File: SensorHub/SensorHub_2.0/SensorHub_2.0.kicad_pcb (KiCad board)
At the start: 2 copper layers, 1 part, among them U1 R7FA4E2B93CFM#AA0

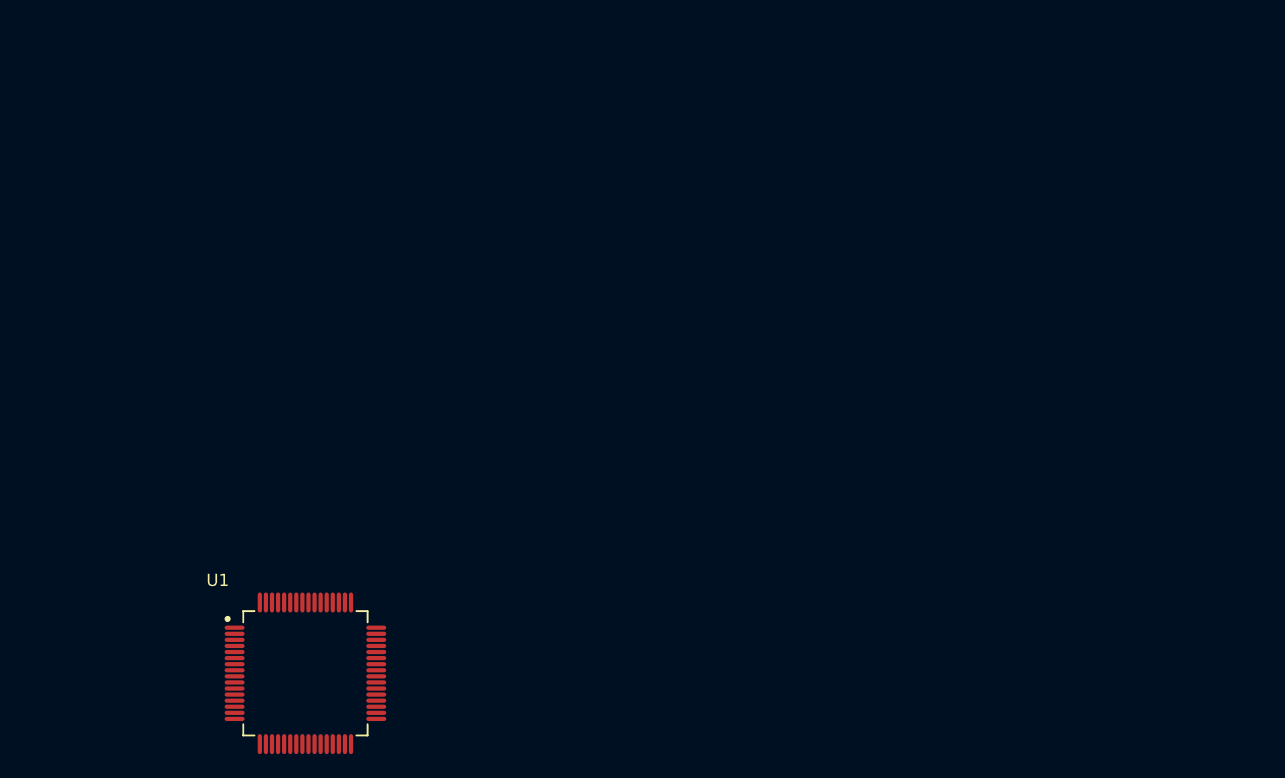
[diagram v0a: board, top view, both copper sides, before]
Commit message: 1st version SensorHub
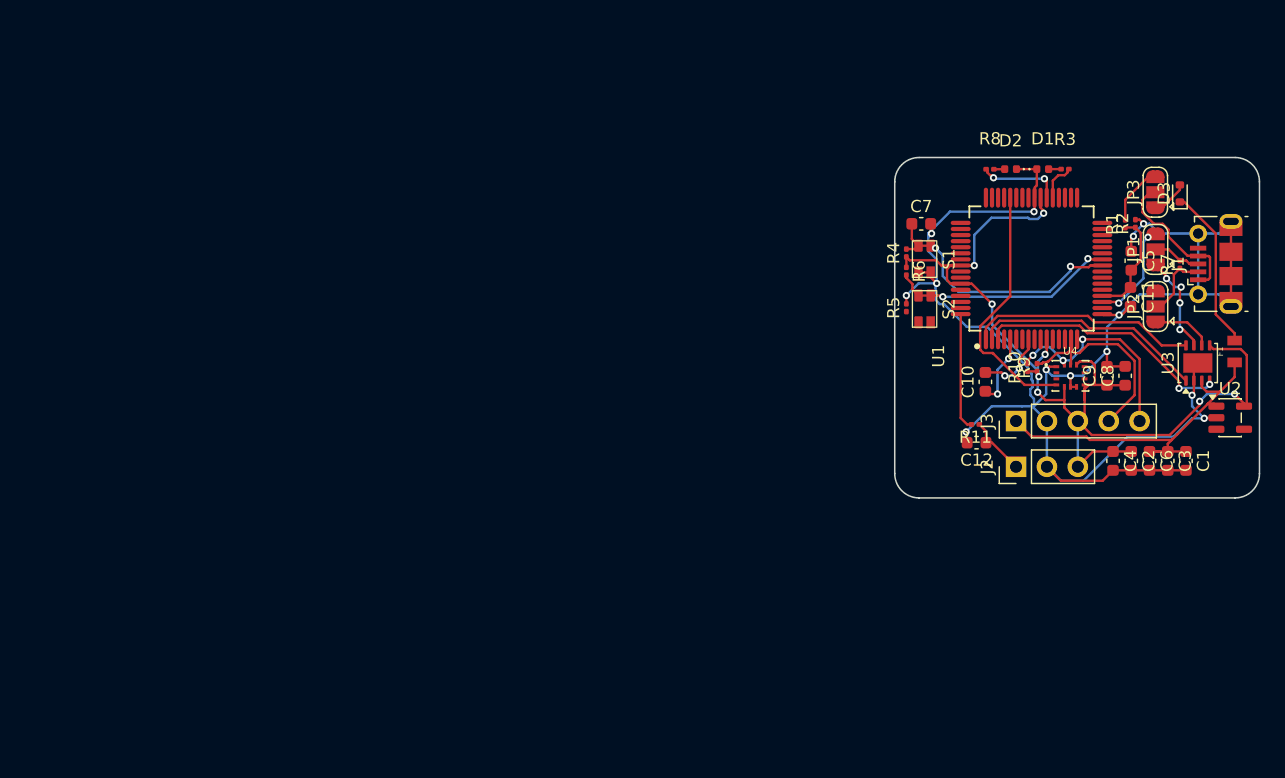
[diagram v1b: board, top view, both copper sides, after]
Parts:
- added C1: 10 uF, Capacitor_SMD:C_0603_1608Metric, F.Cu at (200.5, 120.0)
- added C10: 4.7 uF, Capacitor_SMD:C_0603_1608Metric, F.Cu at (184.0, 113.5)
- added C11: 0.1 uF, Capacitor_SMD:C_0603_1608Metric, F.Cu at (195.9, 106.5)
- added C12: 0.1 uF, Capacitor_SMD:C_0603_1608Metric, F.Cu at (183.3, 118.5)
- added C2: 10 uF, Capacitor_SMD:C_0603_1608Metric, F.Cu at (196.0, 120.0)
- added C3: 1 milF, Capacitor_SMD:C_0603_1608Metric, F.Cu at (199.0, 120.0)
- added C4: 1 milF, Capacitor_SMD:C_0603_1608Metric, F.Cu at (194.5, 120.0)
- added C5: 1 uF, Capacitor_SMD:C_0603_1608Metric, F.Cu at (196.0, 103.5)
- added C6: 0.1 uF, Capacitor_SMD:C_0603_1608Metric, F.Cu at (197.5, 120.0)
- added C7: 1 uF, Capacitor_SMD:C_0603_1608Metric, F.Cu at (178.7, 100.5)
- added C8: 0.1 uF, Capacitor_SMD:C_0603_1608Metric, F.Cu at (195.5, 113.0)
- added C9: 0.1 uF, Capacitor_SMD:C_0603_1608Metric, F.Cu at (194.0, 113.0)
- added D1: LED, LED_SMD:LED_0402_1005Metric, F.Cu at (188.7, 96.0)
- added D2: LED, LED_SMD:LED_0402_1005Metric, F.Cu at (186.1, 96.0)
- added D3: 1N4148WT, Diode_SMD:D_SOD-523, F.Cu at (200.0, 98.0)
- added F1: 6V 0.5A, SensorHub MicroMod Carrier v1.1.0b:0805, F.Cu at (204.5, 111.0)
- added J1: USB_B_Micro, Connector_USB:USB_Micro-B_Molex-105017-0001, F.Cu at (203.0, 103.8)
- added J2: Conn_01x03, Connector_PinHeader_2.54mm:PinHeader_1x03_P2.54mm_Vertical, F.Cu at (186.5, 120.5)
- added J3: Conn_01x05, Connector_PinHeader_2.54mm:PinHeader_1x05_P2.54mm_Vertical, F.Cu at (186.5, 116.7)
- added JP1: SolderJumper_3_Open, Jumper:SolderJumper-3_P1.3mm_Open_RoundedPad1.0x1.5mm, F.Cu at (198.0, 102.6)
- added JP2: SolderJumper_3_Open, Jumper:SolderJumper-3_P1.3mm_Open_RoundedPad1.0x1.5mm, F.Cu at (198.0, 107.3)
- added JP3: SolderJumper_3_Open, Jumper:SolderJumper-3_P1.3mm_Open_RoundedPad1.0x1.5mm, F.Cu at (198.0, 97.9)
- added R1: 15 K, Resistor_SMD:R_0201_0603Metric, F.Cu at (195.5, 100.5)
- added R10: 4.7 K, Resistor_SMD:R_0201_0603Metric, F.Cu at (187.5, 112.3)
- added R11: 1 K, Resistor_SMD:R_0201_0603Metric, F.Cu at (183.2, 117.0)
- added R2: 30 K, Resistor_SMD:R_0201_0603Metric, F.Cu at (196.3, 100.5)
- added R3: 1.33 K, Resistor_SMD:R_0201_0603Metric, F.Cu at (190.6, 96.0)
- added R4: 4.7 K, Resistor_SMD:R_0201_0603Metric, F.Cu at (177.5, 102.9)
- added R5: 1.5 K, Resistor_SMD:R_0201_0603Metric, F.Cu at (177.5, 107.4)
- added R6: 10 K, Resistor_SMD:R_0201_0603Metric, F.Cu at (177.5, 104.4)
- added R7: ~, Resistor_SMD:R_0201_0603Metric, F.Cu at (200.0, 103.8)
- added R8: 1.33 K, Resistor_SMD:R_0201_0603Metric, F.Cu at (184.4, 96.0)
- added R9: 4.7 K, Resistor_SMD:R_0201_0603Metric, F.Cu at (188.2, 112.3)
- added S1: Reset, Library:Button_Mini_2.5x1.7mm, F.Cu at (178.5, 103.4)
- added S2: Boot, Library:Button_Mini_2.5x1.7mm, F.Cu at (178.5, 107.5)
- added U$40: ROBOTPATIENT_SMALL_MODULEBOARD, RobotPatient_BMI270_v1.2_Feb2024:RP_SMALL_SENSOR_OUTLINE, F.Cu at (191.5, 109.0)
- added U2: AP2112K-3.3, Package_TO_SOT_SMD:SOT-23-5, F.Cu at (204.1, 116.5)
- added U3: TJA1051TK-3, Package_SON:HVSON-8-1EP_3x3mm_P0.65mm_EP1.6x2.4mm, F.Cu at (201.5, 112.0)
- added U4: BMI270, BMI270:XDCR_BMI270, F.Cu at (191.0, 113.0)
- moved U1 68.4 mm to (187.8, 104.2), turned to 90 degrees
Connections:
- U1 pad 1: unconnected-(U1-P400-Pad1) -> /Sleep
- U1 pad 11: unconnected-(U1-VCC-Pad11) -> +3.3V
- U1 pad 15: unconnected-(U1-P408-Pad15) -> /SCX
- U1 pad 16: unconnected-(U1-P407-Pad16) -> /SDX
- U1 pad 17: unconnected-(U1-VSS_USB-Pad17) -> GND
- U1 pad 18: unconnected-(U1-USB_DM-Pad18) -> /USB_DM
- U1 pad 19: unconnected-(U1-USB_DP-Pad19) -> /USB_DP
- U1 pad 2: unconnected-(U1-P401-Pad2) -> /TXD
- U1 pad 20: unconnected-(U1-VCC_USB-Pad20) -> /V_USB_Mic
- U1 pad 25: unconnected-(U1-~{RES}-Pad25) -> /RES
- U1 pad 26: unconnected-(U1-MD-Pad26) -> /Boot
- U1 pad 3: unconnected-(U1-CACREF-Pad3) -> /RXD
- U1 pad 37: unconnected-(U1-P112-Pad37) -> /P112
- U1 pad 38: unconnected-(U1-P113-Pad38) -> /P113
- U1 pad 39: unconnected-(U1-VCC-Pad39) -> +3.3V
- U1 pad 40: unconnected-(U1-VSS-Pad40) -> GND
- U1 pad 44: unconnected-(U1-P104-Pad44) -> /INT1
- U1 pad 5: unconnected-(U1-VCL-Pad5) -> /VCL
- U1 pad 56: unconnected-(U1-VREFH-Pad56) -> +3.3V
- U1 pad 59: unconnected-(U1-VREFH0-Pad59) -> +3.3V
- U1 pad 64: unconnected-(U1-P000-Pad64) -> /P000
- U1 pad 8: unconnected-(U1-VSS-Pad8) -> GND
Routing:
- net GND: track 0.00 -> 147.5 mm, vias 0 -> 15
- net +3.3V: track 0.00 -> 87.1 mm, vias 0 -> 8
- net +5V: track 0.00 -> 29.9 mm
- net /RES: track 0.00 -> 22.8 mm, vias 0 -> 2
- net /RXD: track 0.00 -> 21.3 mm, vias 0 -> 2
- net /INT1: track 0.00 -> 21.0 mm
- net /TXD: track 0.00 -> 19.2 mm
- net /SCX: track 0.00 -> 19.1 mm
- net /Sleep: track 0.00 -> 18.8 mm
- net /Boot: track 0.00 -> 18.7 mm, vias 0 -> 2
- net /SDX: track 0.00 -> 18.2 mm, vias 0 -> 3
- net Net-(D3-K): track 0.00 -> 13.5 mm
- net /V_usb: track 0.00 -> 12.9 mm
- net /P000: track 0.00 -> 9.65 mm
- net /V_USB_Mic: track 0.00 -> 8.91 mm
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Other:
- board outline added: 30 x 28 mm

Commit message: MYRGM080200C41RA
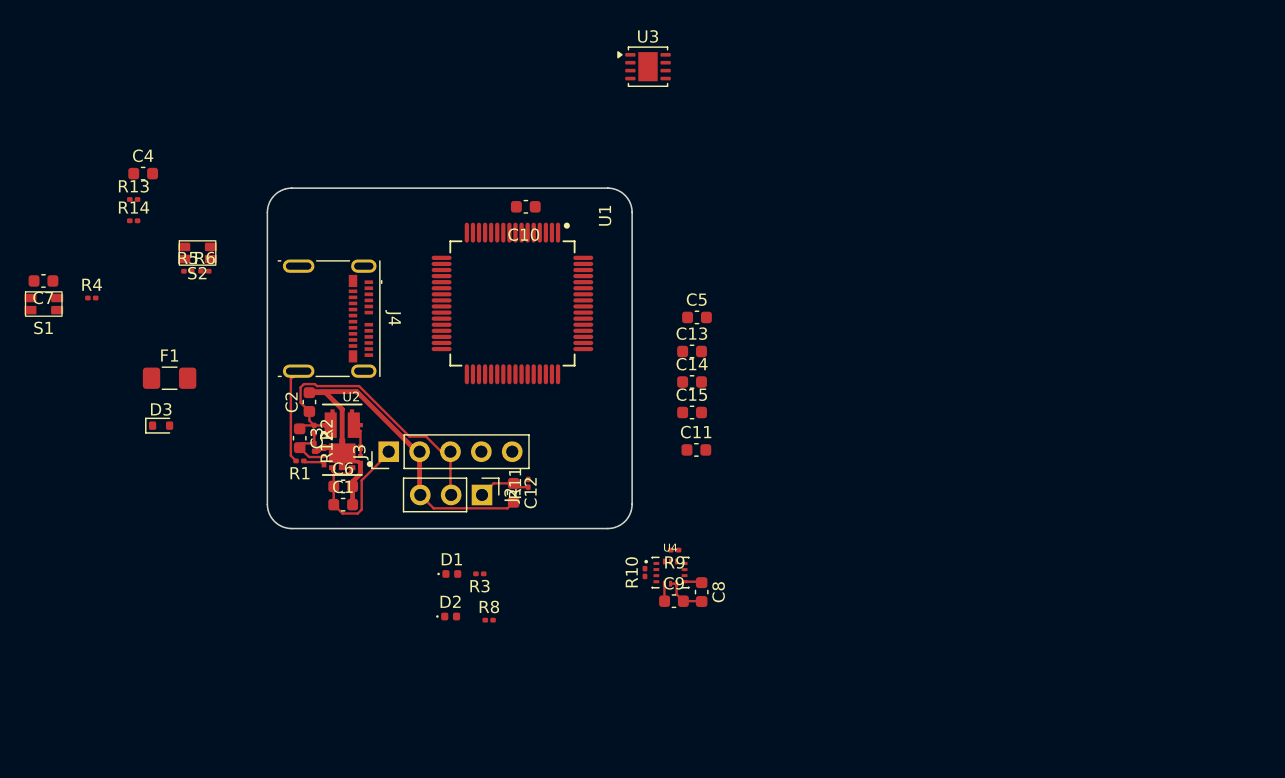
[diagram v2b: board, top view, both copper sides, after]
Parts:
- removed J1: USB_B_Micro, Connector_USB:USB_Micro-B_Molex-105017-0001
- removed JP1, JP2, JP3: SolderJumper_3_Open, Jumper:SolderJumper-3_P1.3mm_Open_RoundedPad1.0x1.5mm
- removed R7: ~, Resistor_SMD:R_0201_0603Metric
- added C13: 0.1 uF, Capacitor_SMD:C_0603_1608Metric, F.Cu at (159.9, 111.0)
- added C14: 0.1 uF, Capacitor_SMD:C_0603_1608Metric, F.Cu at (159.9, 113.5)
- added C15: 0.1 uF, Capacitor_SMD:C_0603_1608Metric, F.Cu at (159.9, 116.0)
- added J4: USB_C_Receptacle, Connector_USB:USB_C_Receptacle_Molex_105450-0101, F.Cu at (130.1, 108.3)
- added R12: 15 K, Resistor_SMD:R_0201_0603Metric, F.Cu at (128.8, 118.9)
- added R13: ~, Resistor_SMD:R_0201_0603Metric, F.Cu at (113.9, 98.5)
- added R14: ~, Resistor_SMD:R_0201_0603Metric, F.Cu at (113.9, 100.2)
- C1, C2: value 10 uF -> 10V/22uF
- C3: value 1 milF -> 330 pF
- C4: value 1 milF -> 50 nF
- C5: value 1 uF -> 0.1 uF
- C6: value 0.1 uF -> 16V/1uF
- F1: footprint SensorHub MicroMod Carrier v1.1.0b:0805 -> Fuse:Fuse_1206_3216Metric_Pad1.42x1.75mm_HandSolder
- R1: value 15 K -> 10 K
- R2: value 30 K -> 47 K
- U2: value AP2112K-3.3 -> MYRGM080200C41RA; footprint Package_TO_SOT_SMD:SOT-23-5 -> MYRGM080200C41RA:MURATA_MYRGM080200C41RA_0
- moved F1 87.6 mm to (116.9, 113.2), turned to 0 degrees
- moved D3 85.9 mm to (116.2, 117.1), turned to 0 degrees
- moved C4 83.2 mm to (114.7, 96.4), turned to 0 degrees
- moved U2 73.1 mm to (131.1, 118.3)
- moved C7 72.4 mm to (106.5, 105.2), turned to 180 degrees
- moved S1 72.0 mm to (106.5, 106.6), turned to 0 degrees
- moved C3 71.4 mm to (127.6, 118.1)
- moved R1 70.6 mm to (127.6, 120.0), turned to 180 degrees
- moved R2 69.6 mm to (128.8, 117.4), turned to -90 degrees
- moved C1 69.4 mm to (131.2, 123.6), turned to 0 degrees
- moved C2 67.8 mm to (128.4, 115.2), turned to 90 degrees
- moved R4 67.1 mm to (110.5, 106.6), turned to 0 degrees
- moved C6 66.4 mm to (131.2, 122.1), turned to 0 degrees
- moved S2 59.5 mm to (119.2, 102.4), turned to 0 degrees
- moved R5 59.2 mm to (118.4, 104.4), turned to 0 degrees
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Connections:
- C11 pad 1: /V_USB_Mic -> +3.3V
- C3 pad 1: +5V -> +3.3V
- C3 pad 2: GND -> /FB
- C4 pad 1: +3.3V -> Net-(C4-Pad1)
- C5 pad 1: GND -> +3.3V
- C5 pad 2: /V_USB_Mic -> GND
- J2 pad 2: GND -> +3.3V
- J2 pad 3: +3.3V -> GND
- R1 pad 1: /V_USB_Mic -> /Sleep
- R1 pad 2: /V_USB_Mic_inp -> GND
- R2 pad 1: /V_USB_Mic -> +3.3V
- R2 pad 2: GND -> /FB
- U1 pad 1: /Sleep -> unconnected-(U1-P400-Pad1)
- U1 pad 20: /V_USB_Mic -> +3.3V
- U1 pad 34: unconnected-(U1-CLKOUT-Pad34) -> /P109 / TXD9
- U2 pad 1: +5V -> unconnected-(U2-1_NC-Pad1)
- U2 pad 2: GND -> /LX
- U2 pad 3: +5V -> /LX
- U2 pad 5: +3.3V -> /FB
- U3 pad 8: /Sleep -> unconnected-(U3-S-Pad8)
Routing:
- net GND: track 147.5 -> 49.4 mm, vias 15 -> 0
- net +3.3V: track 87.1 -> 27.6 mm, vias 8 -> 0
- net /RES: track 22.8 -> 0.00 mm, vias 2 -> 0
- net /RXD: track 21.3 -> 0.00 mm, vias 2 -> 0
- net /INT1: track 21.0 -> 0.00 mm
- net /TXD: track 19.2 -> 0.00 mm
- net /SCX: track 19.1 -> 0.00 mm
- net /Boot: track 18.7 -> 0.00 mm, vias 2 -> 0
- net /SDX: track 18.2 -> 0.00 mm, vias 3 -> 0
- net /Sleep: track 18.8 -> 1.77 mm
- net +5V: track 29.9 -> 13.3 mm
- net Net-(D3-K): track 13.5 -> 0.00 mm
- net /V_usb: track 12.9 -> 0.00 mm
- net /P000: track 9.65 -> 0.00 mm
- net /V_USB_Mic: track 8.91 -> 0.00 mm
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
